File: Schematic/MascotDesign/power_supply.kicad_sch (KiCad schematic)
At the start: 7 parts, among them J1 Charger input, J2 LCD power USB, J3 LCD power USB, J4 PI power USB, U1 Generic_Buck_Regulator, U2 Generic_Buck_Regulator

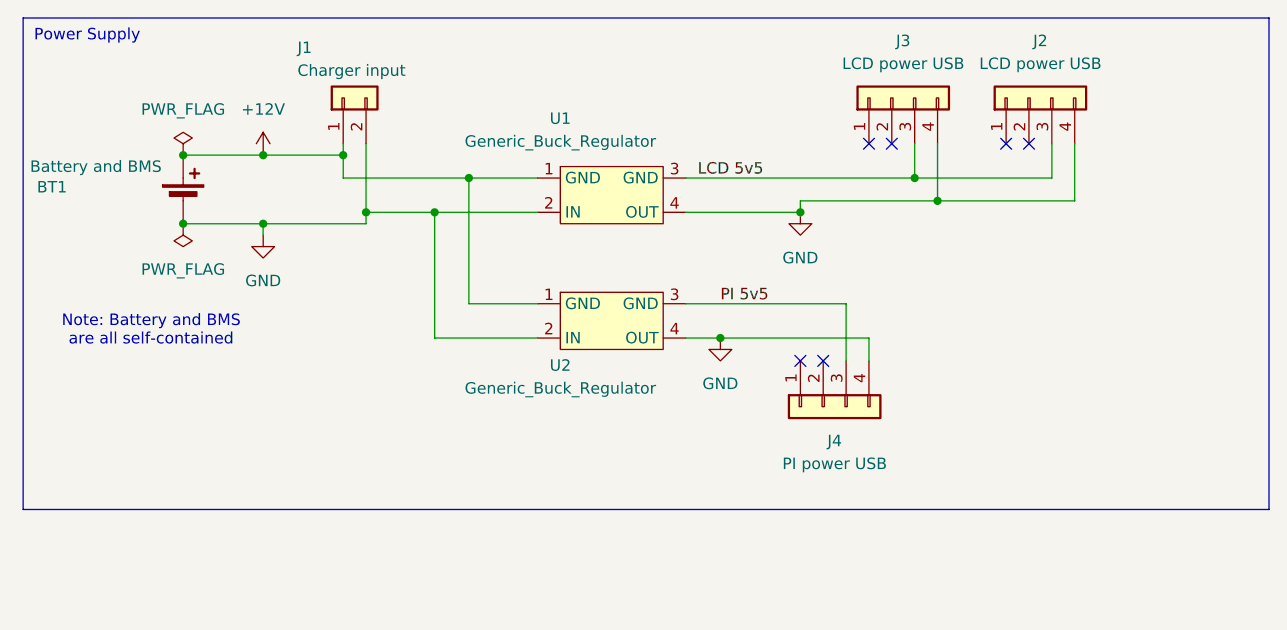
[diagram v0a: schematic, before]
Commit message: Work on power supply schematic
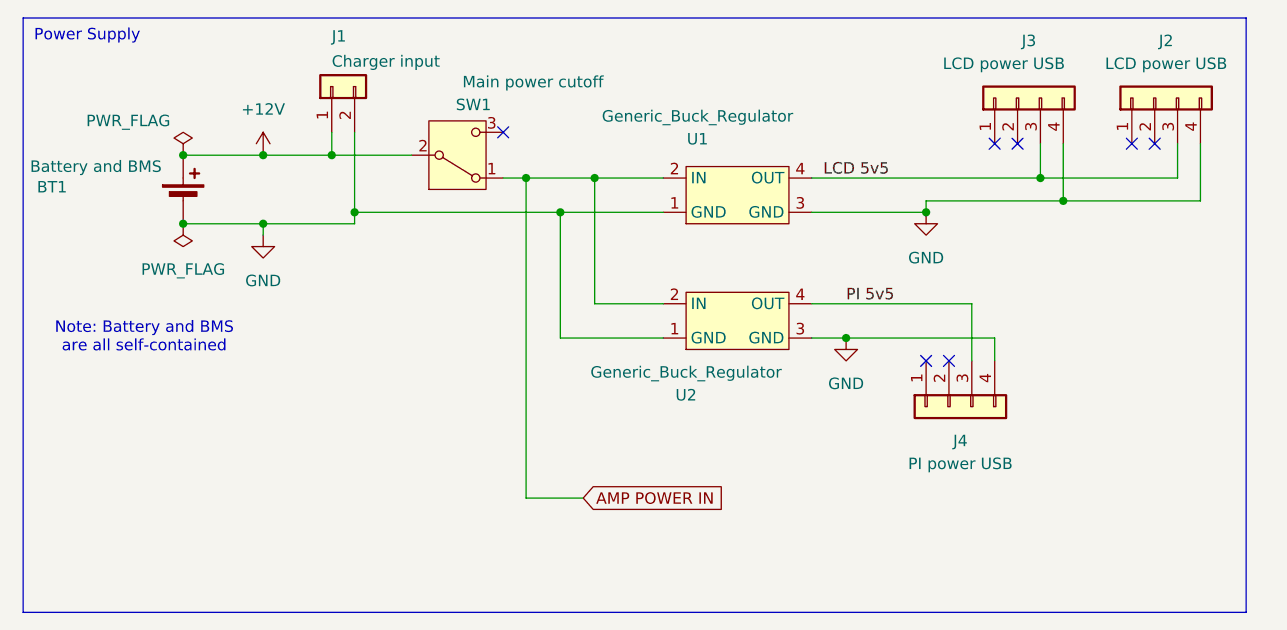
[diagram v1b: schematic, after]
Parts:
- added SW1: Main power cutoff, symbol Switch:SW_SPDT
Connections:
- net +12V: now also SW1.2 (B); no longer U1.1 (GND), U2.1 (GND)
- net GND: now also U1.1 (GND), U1.3 (GND), U2.1 (GND), U2.3 (GND); no longer U1.2 (IN), U1.4 (OUT), U2.2 (IN), U2.4 (OUT)
- net LCD 5v5: now also U1.4 (OUT); no longer U1.3 (GND)
- net PI 5v5: now also U2.4 (OUT); no longer U2.3 (GND)
- new net AMP POWER IN: SW1.1 (A), U1.2 (IN), U2.2 (IN)
- no-connect marks 6 -> 7
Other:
- moved on the sheet: J1, J2, J3, J4, U1, U2
